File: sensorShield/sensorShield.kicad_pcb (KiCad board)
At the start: 2 copper layers, 68.6 x 53.3 mm, 8 parts, among them P1 Power, P2 Analog, P3 Digital, P4 Digital, P5 CONN_01X01, P6 CONN_01X01, P7 CONN_01X01, P8 CONN_01X01

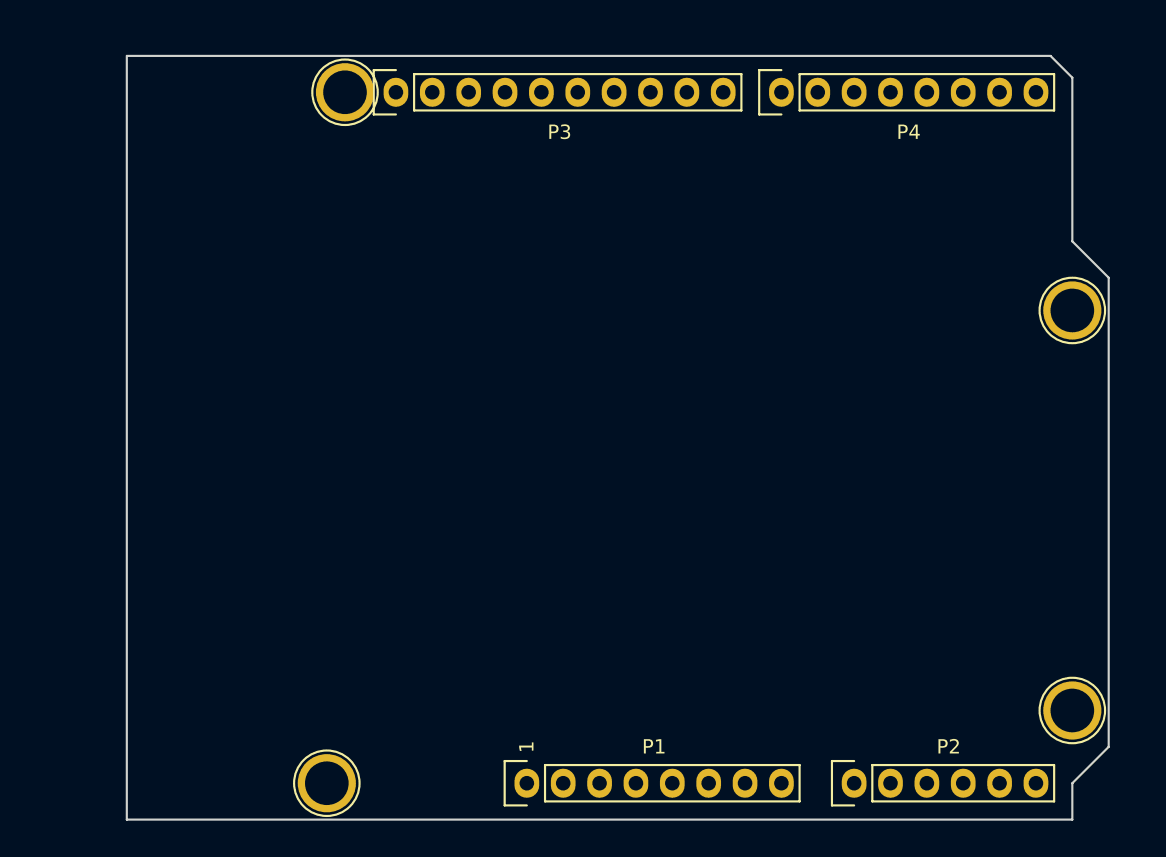
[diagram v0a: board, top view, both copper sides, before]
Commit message: KiCad push
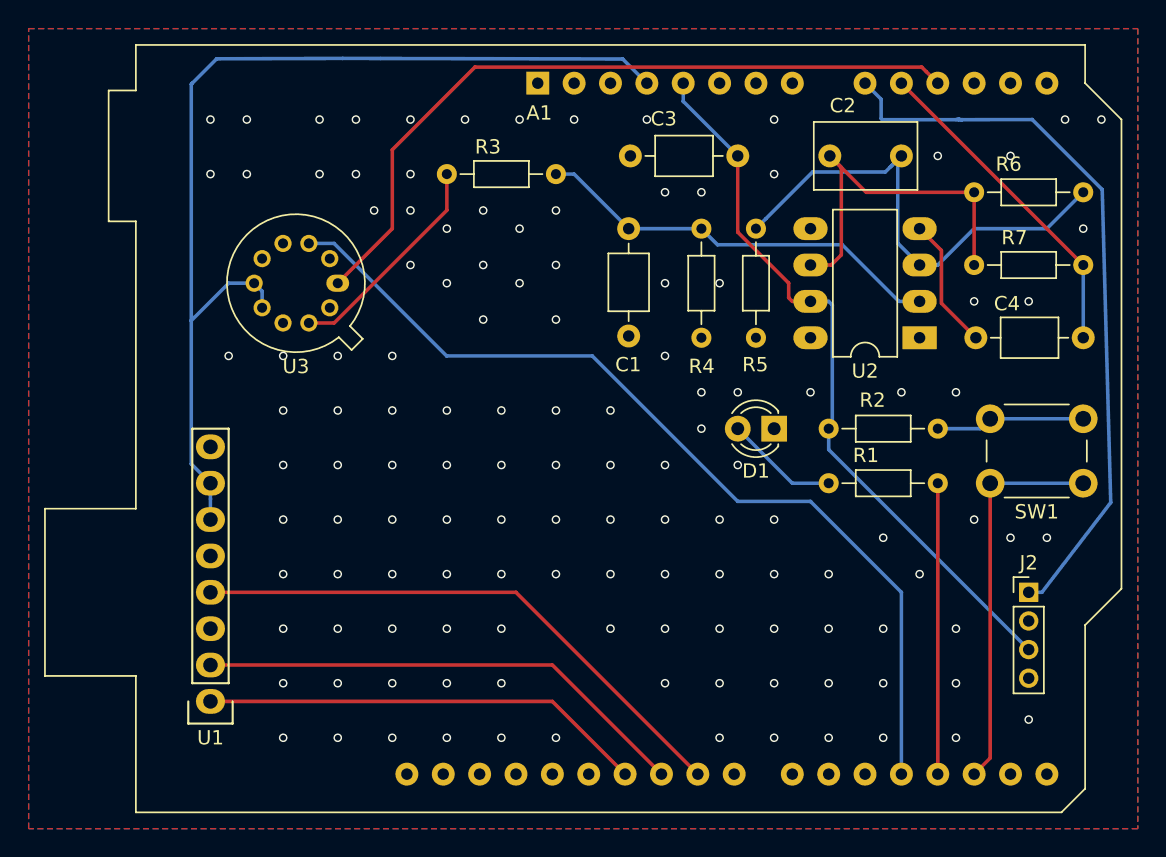
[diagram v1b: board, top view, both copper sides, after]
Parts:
- removed P1: Power, Socket_Arduino_Uno:Socket_Strip_Arduino_1x08
- removed P2: Analog, Socket_Arduino_Uno:Socket_Strip_Arduino_1x06
- removed P3: Digital, Socket_Arduino_Uno:Socket_Strip_Arduino_1x10
- removed P4: Digital, Socket_Arduino_Uno:Socket_Strip_Arduino_1x08
- removed P5, P6, P7, P8: CONN_01X01, Socket_Arduino_Uno:Arduino_1pin
- added A1: Arduino_UNO_R3, Module:Arduino_UNO_R3, F.Cu at (139.7, 74.9)
- added C1: 100n, Capacitor_THT:C_Axial_L3.8mm_D2.6mm_P7.50mm_Horizontal, F.Cu at (146.1, 85.1)
- added C2: 1µ, Capacitor_THT:C_Rect_L7.0mm_W4.5mm_P5.00mm, F.Cu at (165.1, 80.0)
- added C3: 100n, Capacitor_THT:C_Axial_L3.8mm_D2.6mm_P7.50mm_Horizontal, F.Cu at (153.7, 80.0)
- added C4: 100n, Capacitor_THT:C_Axial_L3.8mm_D2.6mm_P7.50mm_Horizontal, F.Cu at (177.8, 92.7)
- added D1: LED, LED_THT:LED_D3.0mm, F.Cu at (156.2, 99.1)
- added J2: GrooveGasSensor, Connector_PinHeader_2.00mm:PinHeader_1x04_P2.00mm_Vertical, F.Cu at (174.0, 110.5)
- added R1: 10k, Resistor_THT:R_Axial_DIN0204_L3.6mm_D1.6mm_P7.62mm_Horizontal, F.Cu at (167.6, 99.1)
- added R2: 330, Resistor_THT:R_Axial_DIN0204_L3.6mm_D1.6mm_P7.62mm_Horizontal, F.Cu at (160.0, 102.9)
- added R3: 10k, Resistor_THT:R_Axial_DIN0204_L3.6mm_D1.6mm_P7.62mm_Horizontal, F.Cu at (141.0, 81.3)
- added R4: 100k, Resistor_THT:R_Axial_DIN0204_L3.6mm_D1.6mm_P7.62mm_Horizontal, F.Cu at (151.1, 92.7)
- added R5: 1k, Resistor_THT:R_Axial_DIN0204_L3.6mm_D1.6mm_P7.62mm_Horizontal, F.Cu at (154.9, 92.7)
- added R6: 100k, Resistor_THT:R_Axial_DIN0204_L3.6mm_D1.6mm_P7.62mm_Horizontal, F.Cu at (170.2, 82.5)
- added R7: 1k, Resistor_THT:R_Axial_DIN0204_L3.6mm_D1.6mm_P7.62mm_Horizontal, F.Cu at (177.8, 87.6)
- added SW1: SW_Push, Button_Switch_THT:SW_PUSH_6mm, F.Cu at (177.8, 102.9)
- added U1: RN2483A, Socket_Arduino_Uno:Socket_Strip_Arduino_1x08, F.Cu at (116.8, 118.1)
- added U2: LTC1050, Package_DIP:DIP-8_W7.62mm_LongPads, F.Cu at (166.4, 92.7)
- added U3: GazSensor, lib:TO-5-10, F.Cu at (125.7, 88.9)
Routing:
- net +3V3: track 0.00 -> 71.6 mm
- net RChauff: track 0.00 -> 64.2 mm
- net CapTemp: track 0.00 -> 51.9 mm
- net +5V: track 0.00 -> 51.7 mm
- net A0: track 0.00 -> 51.6 mm
- net RST: track 0.00 -> 39.3 mm
- net Net-(C2-Pad1): track 0.00 -> 35.3 mm
- net Rx: track 0.00 -> 34.7 mm
- net Tx: track 0.00 -> 31.1 mm
- net Net-(C1-Pad1): track 0.00 -> 29.1 mm
- net D2: track 0.00 -> 27.3 mm
- net Net-(C2-Pad2): track 0.00 -> 25.9 mm
- net A1: track 0.00 -> 23.0 mm
- net D3: track 0.00 -> 20.3 mm
- net Rsensor: track 0.00 -> 15.4 mm
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- added copper zone on B.Cu, net GND
- added copper zone on F.Cu, net GND
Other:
- board outline removed
- board text added: "Emile Sebastianutti Etienne De Prémare ISS 2020-2021"
- board text removed: "1"
